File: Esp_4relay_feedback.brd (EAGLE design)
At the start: 150 x 100 mm, 104 parts, among them IC1 LM1117MP-3.3, IC2 NE555, IC3 7805TV, IC4 7805TV, K1 G5LE, K2 G5LE, K3 G5LE, K4 G5LE, K5 G5LE, K6 G5LE, K7 G5LE, K8 G5LE, Q1 16MHz, Q10 BC547, Q11 TIP120, Q2 BC547, Q4 BC547, Q5 BC547, Q6 BC547, Q7 BC547, Q8 BC547, Q9 BC547, T1 2N7000, T2 2N7000, U2 ATMEGA328P_PDIP

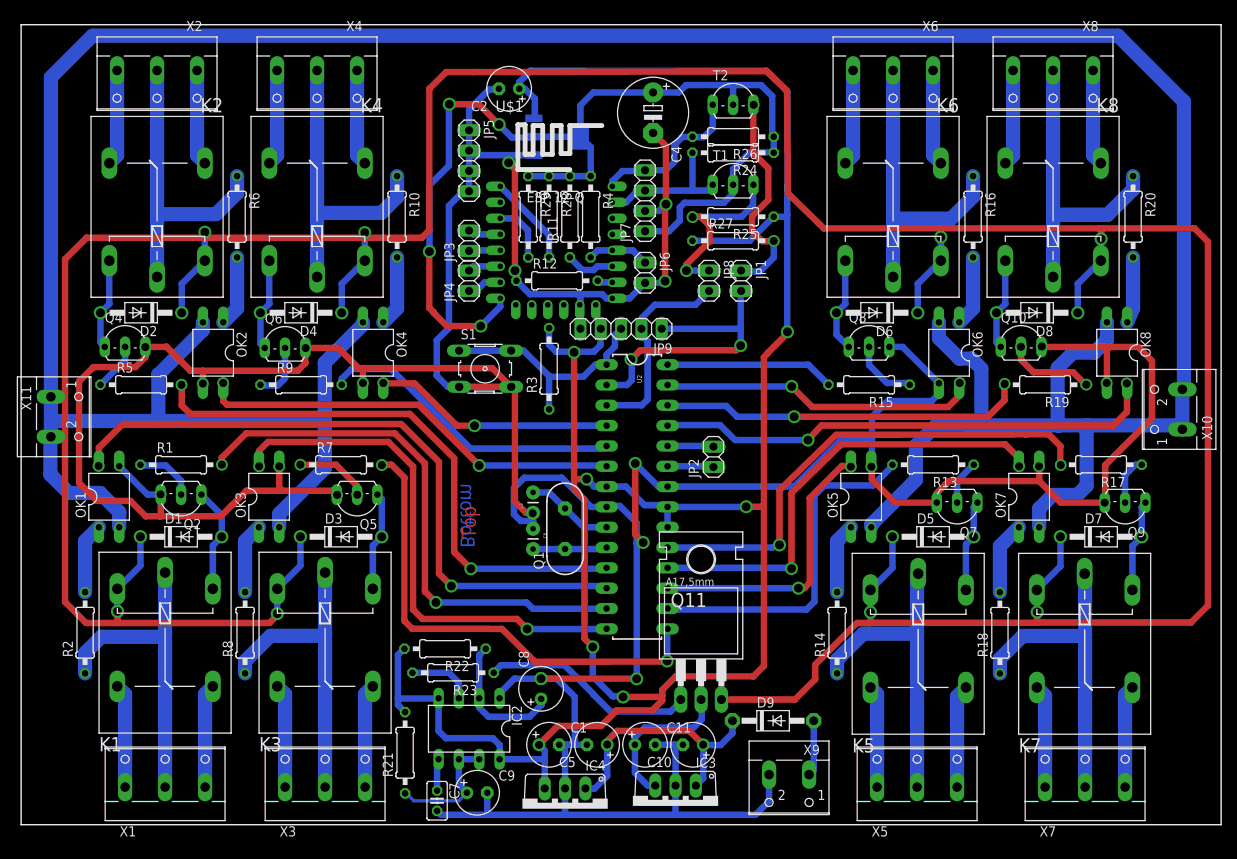
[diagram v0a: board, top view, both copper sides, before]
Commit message: PDF
final pdf added.
developed PCB with this design
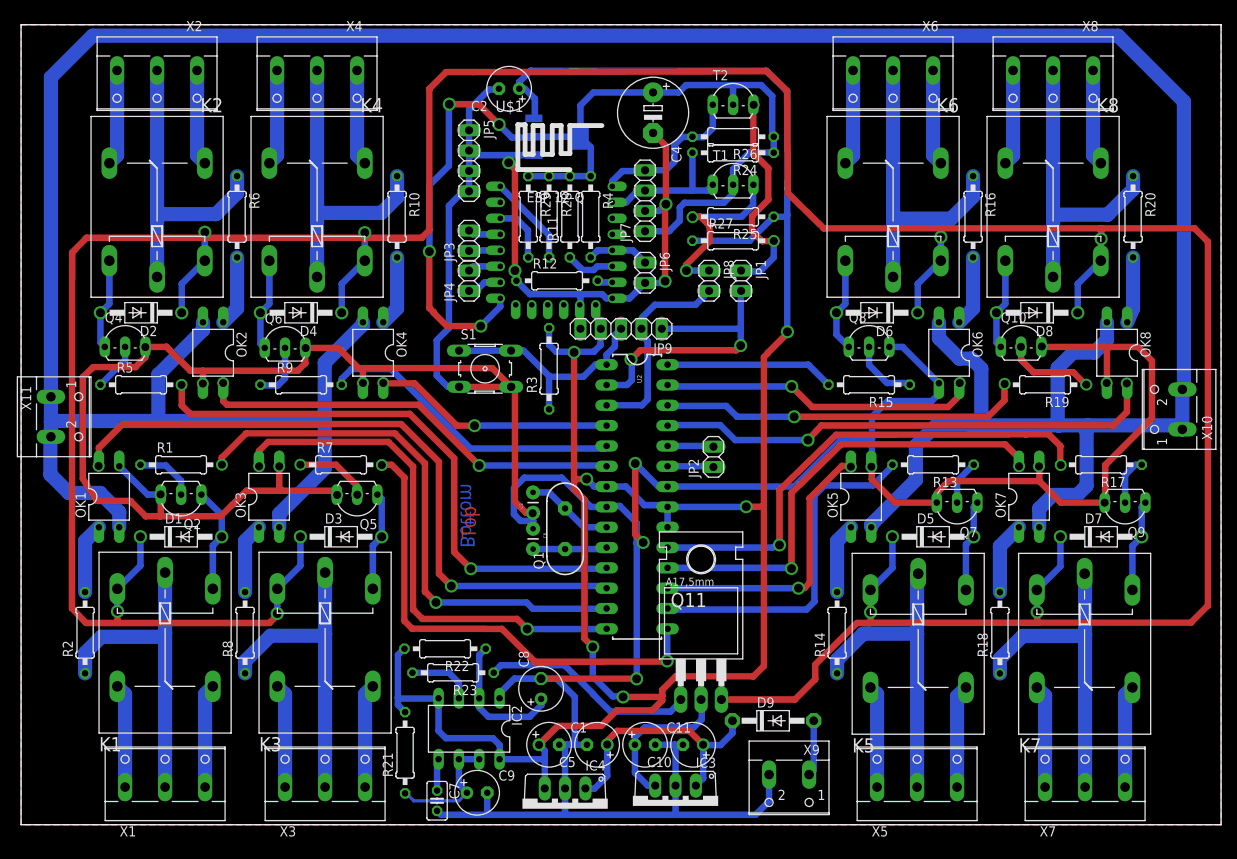
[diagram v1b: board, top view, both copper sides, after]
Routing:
- net RELAY_SUPPLY: track 457.6 -> 456.9 mm
- net GND: track 560.3 -> 559.8 mm
- added copper zone on layer 1, net N$105
- added copper zone on layer 16, net N$106
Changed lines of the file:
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@@
 <setting verticaltext="up"/>
 </settings>
-<grid distance="1" unitdist="mil" unit="mil" style="lines" multiple="1" display="yes" altdistance="1" altunitdist="mm" altunit="mm"/>
+<grid distance="1" unitdist="mm" unit="mm" style="lines" multiple="1" display="yes" altdistance="1" altunitdist="mm" altunit="mm"/>
 <layers>
-<layer number="1" name="Top" color="4" fill="1" visible="yes" active="yes"/>
+<layer number="1" name="Top" color="4" fill="1" visible="no" active="yes"/>
 <layer number="2" name="Route2" color="1" fill="3" visible="no" active="no"/>
 <layer number="3" name="Route3" color="4" fill="3" visible="no" active="no"/>
@@
 <layer number="17" name="Pads" color="2" fill="1" visible="yes" active="yes"/>
 <layer number="18" name="Vias" color="2" fill="1" visible="yes" active="yes"/>
-<layer number="19" name="Unrouted" color="6" fill="1" visible="yes" active="yes"/>
+<layer number="19" name="Unrouted" color="6" fill="1" visible="no" active="yes"/>
 <layer number="20" name="Dimension" color="15" fill="1" visible="yes" active="yes"/>
-<layer number="21" name="tPlace" color="7" fill="1" visible="yes" active="yes"/>
-<layer number="22" name="bPlace" color="7" fill="1" visible="yes" active="yes"/>
-<layer number="23" name="tOrigins" color="15" fill="1" visible="yes" active="yes"/>
-<layer number="24" name="bOrigins" color="15" fill="1" visible="yes" active="yes"/>
-<layer number="25" name="tNames" color="7" fill="1" visible="yes" active="yes"/>
-<layer number="26" name="bNames" color="7" fill="1" visible="yes" active="yes"/>
+<layer number="21" name="tPlace" color="7" fill="1" visible="no" active="yes"/>
+<layer number="22" name="bPlace" color="7" fill="1" visible="no" active="yes"/>
+<layer number="23" name="tOrigins" color="15" fill="1" visible="no" active="yes"/>
+<layer number="24" name="bOrigins" color="15" fill="1" visible="no" active="yes"/>
+<layer number="25" name="tNames" color="7" fill="1" visible="no" active="yes"/>
+<layer number="26" name="bNames" color="7" fill="1" visible="no" active="yes"/>
 <layer number="27" name="tValues" color="7" fill="1" visible="no" active="yes"/>
 <layer number="28" name="bValues" color="7" fill="1" visible="no" active="yes"/>
@@
 <wire x1="118.7196" y1="56.7436" x2="117.1702" y2="56.7436" width="0.8128" layer="1"/>
 <wire x1="122.3518" y1="39.9542" x2="120.9548" y2="38.5572" width="0.8128" layer="1"/>
-<wire x1="103.251" y1="55.4228" x2="105.029" y2="57.2008" width="0.8128" layer="1"/>
+<wire x1="103.7082" y1="55.9562" x2="105.029" y2="57.2008" width="0.8128" layer="1"/>
 <wire x1="105.029" y1="57.2008" x2="110.2868" y2="57.2008" width="0.8128" layer="1"/>
 <wire x1="110.2868" y1="57.2008" x2="111.5314" y2="58.4454" width="0.8128" layer="1"/>
@@
 <wire x1="111.5822" y1="38.5572" x2="109.6518" y2="40.4876" width="0.8128" layer="1"/>
 <wire x1="109.6518" y1="40.4876" x2="105.4862" y2="40.4876" width="0.8128" layer="1"/>
-<wire x1="105.4862" y1="40.4876" x2="103.251" y2="42.7228" width="0.8128" layer="1"/>
-<wire x1="103.251" y1="42.7228" x2="103.251" y2="55.4228" width="0.8128" layer="1"/>
+<wire x1="105.4862" y1="40.4876" x2="103.7082" y2="43.2562" width="0.8128" layer="1"/>
+<wire x1="103.7082" y1="43.2562" x2="103.7082" y2="55.9562" width="0.8128" layer="1"/>
 <wire x1="113.46" y1="41.27" x2="113.46" y2="38.8384" width="0.8128" layer="1"/>
 <wire x1="113.46" y1="38.8384" x2="113.4872" y2="38.8112" width="0.8128" layer="1"/>
@@
 <wire x1="138.938" y1="73.3806" x2="118.999" y2="73.3806" width="0.8128" layer="1"/>
 <wire x1="118.999" y1="73.3806" x2="104.1908" y2="73.3806" width="0.8128" layer="1"/>
-<wire x1="104.1908" y1="73.3806" x2="101.4984" y2="70.6882" width="0.8128" layer="1"/>
-<wire x1="101.4984" y1="70.6882" x2="101.4984" y2="27.8384" width="0.8128" layer="1"/>
-<wire x1="101.4984" y1="27.8384" x2="104.1146" y2="25.2222" width="0.8128" layer="1"/>
+<wire x1="104.1908" y1="73.3806" x2="102.3874" y2="71.5264" width="0.8128" layer="1"/>
+<wire x1="102.3874" y1="71.5264" x2="102.362" y2="27.051" width="0.8128" layer="1"/>
+<wire x1="102.362" y1="27.051" x2="104.1146" y2="25.2222" width="0.8128" layer="1"/>
 <wire x1="104.1146" y1="25.2222" x2="108.204" y2="25.2222" width="0.8128" layer="1"/>
 <wire x1="108.204" y1="25.2222" x2="127.0508" y2="25.2222" width="0.8128" layer="1"/>
@@
 <via x="183.5404" y="15.6718" extent="1-16" drill="1" diameter="1.4224" shape="square"/>
 </signal>
+<signal name="N$105">
+<polygon width="0.4064" layer="1" isolate="1.9304">
+<vertex x="96" y="100"/>
+<vertex x="246" y="100"/>
+<vertex x="246" y="0"/>
+<vertex x="96" y="0"/>
+</polygon>
+</signal>
+<signal name="N$106">
+<polygon width="0.4064" layer="16" isolate="1.9304">
+<vertex x="96" y="100"/>
+<vertex x="246" y="100"/>
+<vertex x="246" y="0"/>
+<vertex x="96" y="0"/>
+</polygon>
+</signal>
 </signals>
